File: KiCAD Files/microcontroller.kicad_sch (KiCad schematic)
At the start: 46 parts, among them IC5 AZ1117IH-3.3TRG1, J3 TSW-103-14-S-D, J4 TSW-103-14-S-D, J7 TSW-105-05-F-S, U1 STM32H7A3RGTx, Y1 ABM8G-48.000MHZ-18-D2Y-T

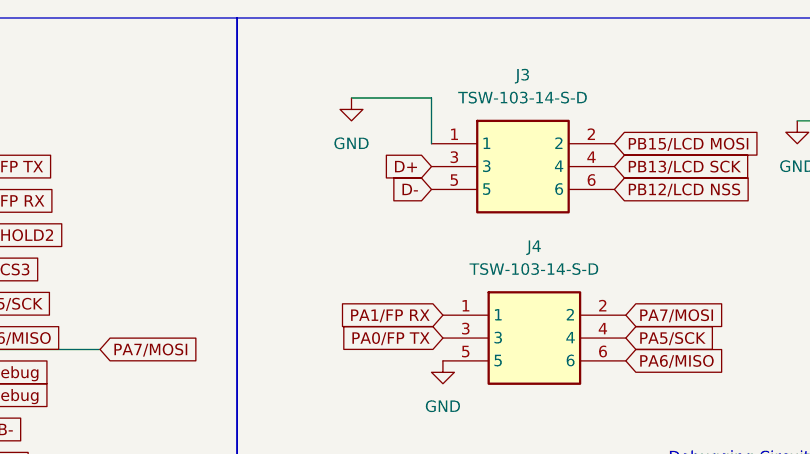
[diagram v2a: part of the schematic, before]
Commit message: made most of the easy changes for the pcb
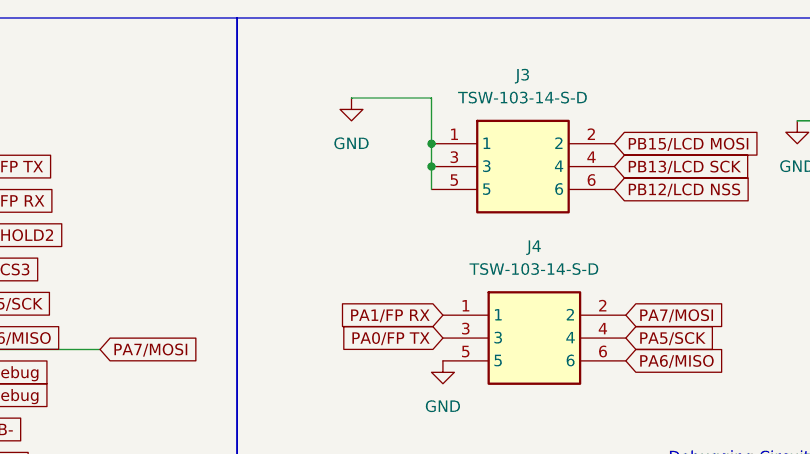
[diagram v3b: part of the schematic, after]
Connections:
- net D+ is gone; now on net GND: J3.3
- net D- is gone; now on net GND: J3.5
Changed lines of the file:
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@@
+	)
+	(junction
+		(at 130.81 26.67)
+		(diameter 0)
+		(color 0 0 0 0)
 	)
 	(junction
@@
 	)
 	(junction
+		(at 130.81 29.21)
+		(diameter 0)
+		(color 0 0 0 0)
+	)
+	(junction
 		(at 45.72 162.56)
 		(diameter 0)
@@
 	(wire
 		(pts
+			(xy 130.81 26.67) (xy 130.81 29.21)
+		)
+		(stroke
+			(width 0)
+			(type default)
+		)
+	)
+	(wire
+		(pts
 			(xy 223.52 83.82) (xy 215.9 83.82)
 		)
@@
 		(pts
 			(xy 76.2 31.75) (xy 77.47 31.75)
+		)
+		(stroke
+			(width 0)
+			(type default)
+		)
+	)
+	(wire
+		(pts
+			(xy 130.81 29.21) (xy 130.81 31.75)
 		)
 		(stroke
@@
 		)
 	)
-	(global_label "D+"
-		(shape input)
-		(at 130.81 29.21 180)
-		(fields_autoplaced yes)
-		(effects
-			(font
-				(size 1.27 1.27)
-				(color 0 0 0 1)
-			)
-			(justify right)
-		)
-		(property "Intersheetrefs" "${INTERSHEET_REFS}"
-			(at 124.9824 29.21 0)
-			(effects
-				(font
-					(size 1.27 1.27)
-				)
-				(justify right)
-				(hide yes)
-			)
-		)
-	)
 	(global_label "PC1{slash}HOLD3"
 		(shape input)
@@
 			(effects
 				(font
-					(size 1.27 1.27)
-				)
-				(justify right)
-				(hide yes)
-			)
-		)
-	)
-	(global_label "D-"
-		(shape input)
-		(at 130.81 31.75 180)
-		(fields_autoplaced yes)
-		(effects
-			(font
-				(size 1.27 1.27)
-				(color 0 0 0 1)
-			)
-			(justify right)
-		)
-		(property "Intersheetrefs" "${INTERSHEET_REFS}"
-			(at 124.9824 31.75 0)
-			(effects
-				(font
